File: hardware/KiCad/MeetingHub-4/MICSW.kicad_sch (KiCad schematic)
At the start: 13 parts, among them K1 Select NB1, K2 Select NB2, K3 Select NB3, K4 Select NB4, SW1 MUTE, SW2 Select NB1, SW3 Select NB2, SW4 Select NB3, SW5 Select NB4

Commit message: jlcpcb production  W2026080810364558  PCB/PCBA
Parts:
- SW1, SW2, SW3, SW4, SW5: footprint Connector_JST:JST_XH_B2B-XH-A_1x02_P2.50mm_Vertical -> MeetingHub-4:SW_SHOUHAN_TS665ZJ
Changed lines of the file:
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@@
       (effects (font (size 1.27 1.27)))
     )
-    (property "Footprint" "Connector_JST:JST_XH_B2B-XH-A_1x02_P2.50mm_Vertical" (at 95.25 39.37 0)
+    (property "Footprint" "MeetingHub-4:SW_SHOUHAN_TS665ZJ" (at 95.25 39.37 0)
       (effects (font (size 1.27 1.27)) hide)
     )
@@
       (effects (font (size 1.27 1.27)))
     )
-    (property "Footprint" "Connector_JST:JST_XH_B2B-XH-A_1x02_P2.50mm_Vertical" (at 59.69 30.48 0)
+    (property "Footprint" "MeetingHub-4:SW_SHOUHAN_TS665ZJ" (at 59.69 30.48 0)
       (effects (font (size 1.27 1.27)) hide)
     )
@@
       (effects (font (size 1.27 1.27)))
     )
-    (property "Footprint" "Connector_JST:JST_XH_B2B-XH-A_1x02_P2.50mm_Vertical" (at 95.25 80.01 0)
+    (property "Footprint" "MeetingHub-4:SW_SHOUHAN_TS665ZJ" (at 95.25 80.01 0)
       (effects (font (size 1.27 1.27)) hide)
     )
@@
       (effects (font (size 1.27 1.27)))
     )
-    (property "Footprint" "Connector_JST:JST_XH_B2B-XH-A_1x02_P2.50mm_Vertical" (at 95.25 160.02 0)
+    (property "Footprint" "MeetingHub-4:SW_SHOUHAN_TS665ZJ" (at 95.25 160.02 0)
       (effects (font (size 1.27 1.27)) hide)
     )
@@
       (effects (font (size 1.27 1.27)))
     )
-    (property "Footprint" "Connector_JST:JST_XH_B2B-XH-A_1x02_P2.50mm_Vertical" (at 95.25 119.38 0)
-      (effects (font (size 1.27 1.27)) hide)
-    )
+    (property "Footprint" "MeetingHub-4:SW_SHOUHAN_TS665ZJ" (at 95.25 119.38 0)
+      (effects (font (size 1.27 1.27)) hide)
+    )

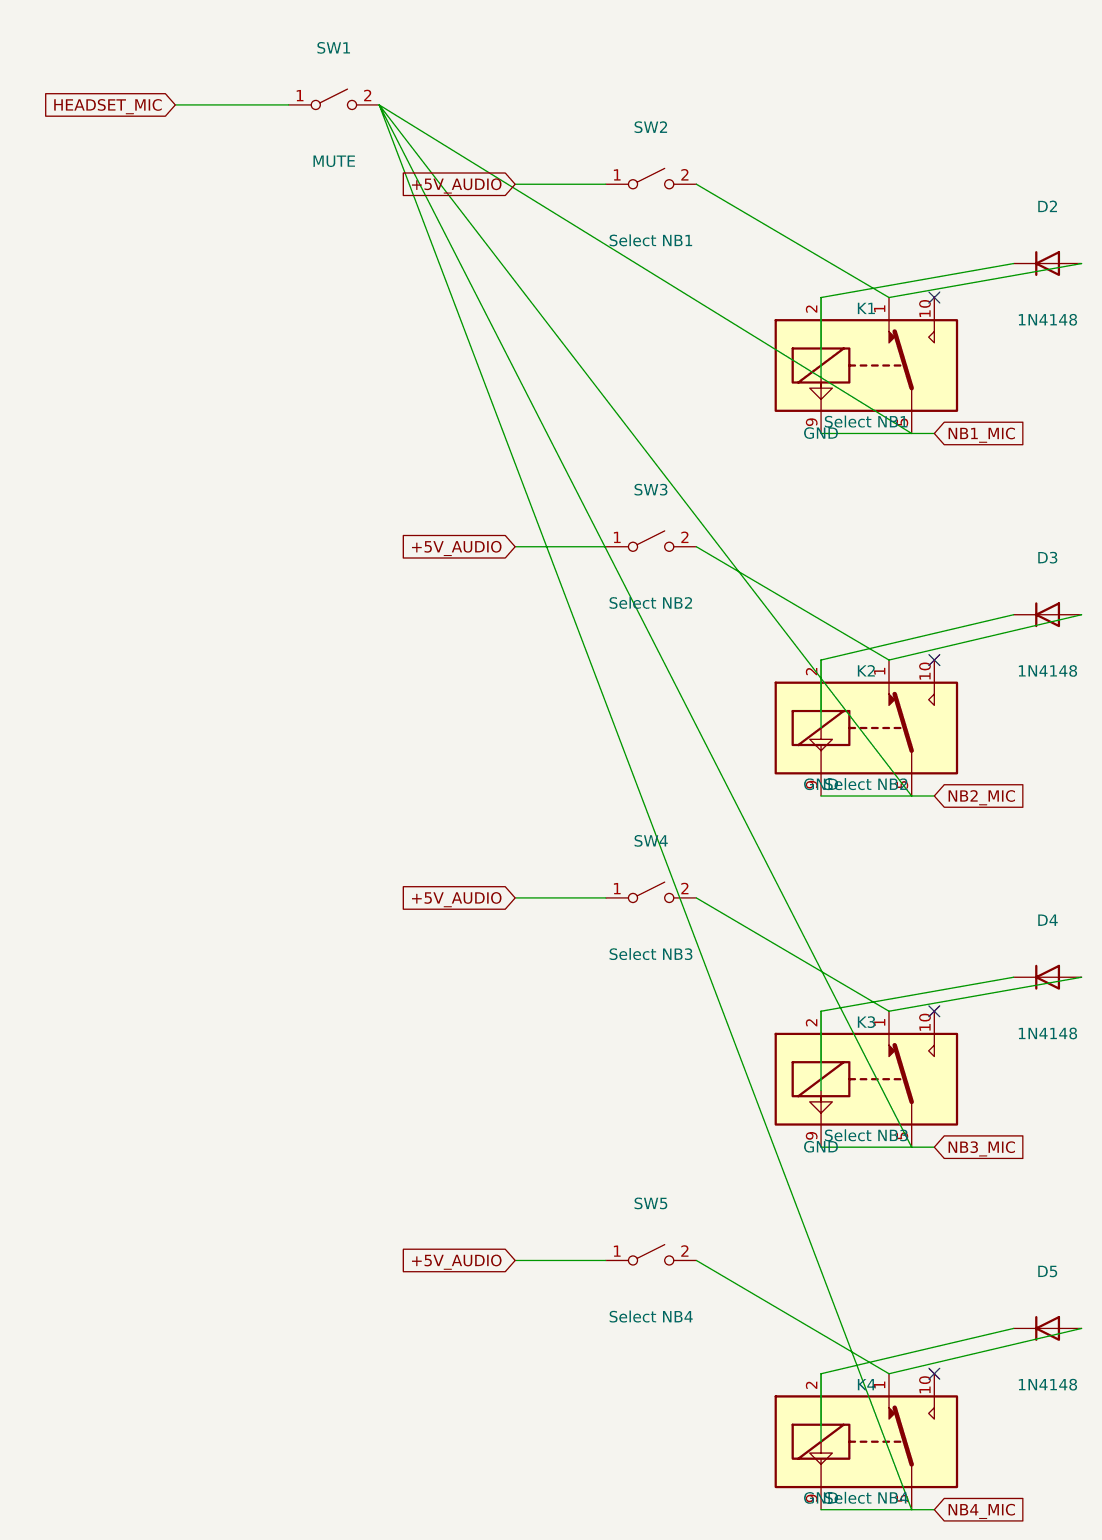
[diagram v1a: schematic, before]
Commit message: Rascunho projeto após fabricação com prblemas
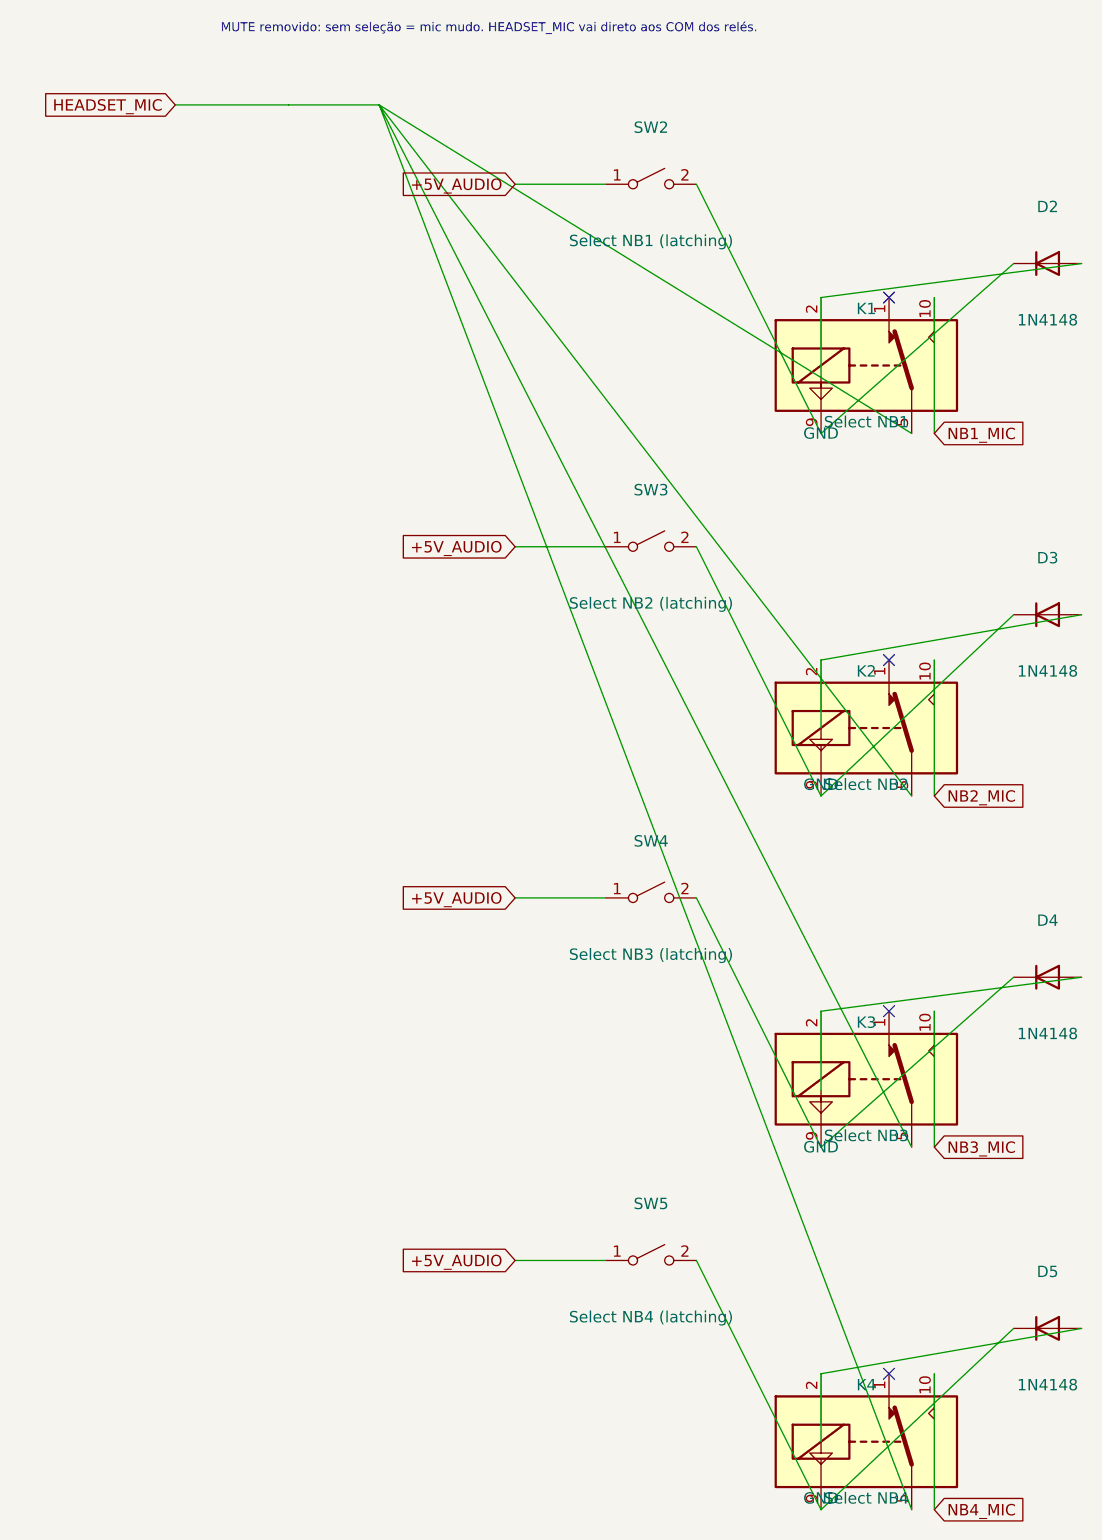
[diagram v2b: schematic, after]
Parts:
- removed SW1: MUTE, MeetingHub-4:SW_SHOUHAN_TS665ZJ, symbol Switch:SW_SPST
- SW2: value Select NB1 -> Select NB1 (latching); footprint MeetingHub-4:SW_SHOUHAN_TS665ZJ -> MeetingHub-4:SW_PushLock_PS-22F03
- SW3: value Select NB2 -> Select NB2 (latching); footprint MeetingHub-4:SW_SHOUHAN_TS665ZJ -> MeetingHub-4:SW_PushLock_PS-22F03
- SW4: value Select NB3 -> Select NB3 (latching); footprint MeetingHub-4:SW_SHOUHAN_TS665ZJ -> MeetingHub-4:SW_PushLock_PS-22F03
- SW5: value Select NB4 -> Select NB4 (latching); footprint MeetingHub-4:SW_SHOUHAN_TS665ZJ -> MeetingHub-4:SW_PushLock_PS-22F03
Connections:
- net GND: now also D2.2 (A), D3.2 (A), D4.2 (A), D5.2 (A); no longer D2.1 (K), D3.1 (K), D4.1 (K), D5.1 (K)
- net HEADSET_MIC: now also K1.5, K1.6, K2.5, K2.6, K3.5, K3.6, K4.5, K4.6
- net NB1_MIC: now also K1.10; no longer K1.9
- net NB2_MIC: now also K2.10; no longer K2.9
- net NB3_MIC: now also K3.10; no longer K3.9
- net NB4_MIC: now also K4.10; no longer K4.9
- new net: D2.1 (K), K1.9, SW2.2 (B)
- new net: D3.1 (K), K2.9, SW3.2 (B)
- new net: D4.1 (K), K3.9, SW4.2 (B)
- new net: D5.1 (K), K4.9, SW5.2 (B)
- now unconnected: K1.1, K2.1, K3.1, K4.1
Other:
- note added: "MUTE removido: sem seleção = mic mudo. HEADSET_MIC vai direto aos COM dos relés."
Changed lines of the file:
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@@
 (kicad_sch (version 20230121) (generator eeschema)
   (paper "A4")
-  (wire (pts (xy 100.33 160.02) (xy 121.92 172.72))
-    (stroke (width 0) (type default))
-  )
-  (no_connect (at 127 52.07))
-  (no_connect (at 127 92.71))
-  (no_connect (at 127 132.08))
-  (no_connect (at 127 172.72))
-  (wire (pts (xy 114.3 107.95) (xy 127 107.95))
-    (stroke (width 0) (type default))
-  )
-  (wire (pts (xy 114.3 187.96) (xy 127 187.96))
-    (stroke (width 0) (type default))
-  )
-  (wire (pts (xy 135.89 87.63) (xy 114.3 92.71))
-    (stroke (width 0) (type default))
-  )
-  (wire (pts (xy 143.51 128.27) (xy 121.92 132.08))
+  (wire (pts (xy 100.33 160.02) (xy 114.3 187.96))
+    (stroke (width 0) (type default))
+  )
+  (no_connect (at 121.92 52.07))
+  (no_connect (at 121.92 92.71))
+  (no_connect (at 121.92 132.08))
+  (no_connect (at 121.92 172.72))
+  (wire (pts (xy 127 92.71) (xy 127 107.95))
+    (stroke (width 0) (type default))
+  )
+  (wire (pts (xy 127 172.72) (xy 127 187.96))
+    (stroke (width 0) (type default))
+  )
+  (wire (pts (xy 135.89 87.63) (xy 114.3 107.95))
+    (stroke (width 0) (type default))
+  )
+  (wire (pts (xy 143.51 128.27) (xy 114.3 132.08))
     (stroke (width 0) (type default))
   )
@@
     (stroke (width 0) (type default))
   )
-  (wire (pts (xy 100.33 39.37) (xy 121.92 52.07))
+  (wire (pts (xy 100.33 39.37) (xy 114.3 67.31))
     (stroke (width 0) (type default))
   )
@@
     (stroke (width 0) (type default))
   )
+  (wire (pts (xy 54.61 30.48) (xy 64.77 30.48))
+    (stroke (width 0) (type default))
+  )
   (wire (pts (xy 114.3 132.08) (xy 114.3 140.97))
     (stroke (width 0) (type default))
@@
     (stroke (width 0) (type default))
   )
-  (wire (pts (xy 114.3 67.31) (xy 127 67.31))
-    (stroke (width 0) (type default))
-  )
-  (wire (pts (xy 114.3 147.32) (xy 127 147.32))
+  (wire (pts (xy 127 52.07) (xy 127 67.31))
+    (stroke (width 0) (type default))
+  )
+  (wire (pts (xy 127 132.08) (xy 127 147.32))
     (stroke (width 0) (type default))
   )
@@
     (stroke (width 0) (type default))
   )
-  (wire (pts (xy 135.89 48.26) (xy 114.3 52.07))
-    (stroke (width 0) (type default))
-  )
-  (wire (pts (xy 143.51 48.26) (xy 121.92 52.07))
-    (stroke (width 0) (type default))
-  )
-  (wire (pts (xy 135.89 128.27) (xy 114.3 132.08))
+  (wire (pts (xy 135.89 48.26) (xy 114.3 67.31))
+    (stroke (width 0) (type default))
+  )
+  (wire (pts (xy 143.51 48.26) (xy 114.3 52.07))
+    (stroke (width 0) (type default))
+  )
+  (wire (pts (xy 135.89 128.27) (xy 114.3 147.32))
     (stroke (width 0) (type default))
   )
@@
     (stroke (width 0) (type default))
   )
-  (wire (pts (xy 100.33 119.38) (xy 121.92 132.08))
-    (stroke (width 0) (type default))
-  )
-  (wire (pts (xy 135.89 167.64) (xy 114.3 172.72))
+  (wire (pts (xy 100.33 119.38) (xy 114.3 147.32))
+    (stroke (width 0) (type default))
+  )
+  (wire (pts (xy 135.89 167.64) (xy 114.3 187.96))
     (stroke (width 0) (type default))
   )
@@
     (stroke (width 0) (type default))
   )
-  (wire (pts (xy 143.51 167.64) (xy 121.92 172.72))
+  (wire (pts (xy 143.51 167.64) (xy 114.3 172.72))
     (stroke (width 0) (type default))
   )
@@
     (stroke (width 0) (type default))
   )
-  (wire (pts (xy 100.33 80.01) (xy 121.92 92.71))
-    (stroke (width 0) (type default))
-  )
-  (wire (pts (xy 143.51 87.63) (xy 121.92 92.71))
+  (wire (pts (xy 100.33 80.01) (xy 114.3 107.95))
+    (stroke (width 0) (type default))
+  )
+  (wire (pts (xy 143.51 87.63) (xy 114.3 92.71))
     (stroke (width 0) (type default))
   )
@@
       (effects (font (size 1.27 1.27)))
     )
-    (property "Value" "Select NB1" (at 95.25 45.72 0)
-      (effects (font (size 1.27 1.27)))
-    )
-    (property "Footprint" "MeetingHub-4:SW_SHOUHAN_TS665ZJ" (at 95.25 39.37 0)
+    (property "Value" "Select NB1 (latching)" (at 95.25 45.72 0)
+      (effects (font (size 1.27 1.27)))
+    )
+    (property "Footprint" "MeetingHub-4:SW_PushLock_PS-22F03" (at 95.25 39.37 0)
       (effects (font (size 1.27 1.27)) hide)
     )
@@
     )
   )
-  (symbol (lib_id "Switch:SW_SPST") (at 59.69 30.48 0) (unit 1)
-    (in_bom yes) (on_board yes) (dnp no)
-    (property "Reference" "SW1" (at 59.69 24.13 0)
-      (effects (font (size 1.27 1.27)))
-    )
-    (property "Value" "MUTE" (at 59.69 36.83 0)
-      (effects (font (size 1.27 1.27)))
-    )
-    (property "Footprint" "MeetingHub-4:SW_SHOUHAN_TS665ZJ" (at 59.69 30.48 0)
-      (effects (font (size 1.27 1.27)) hide)
-    )
-    (property "Datasheet" "" (at 59.69 30.48 0)
-      (effects (font (size 1.27 1.27)) hide)
-    )
-    (pin "1")
-    (pin "2")
-    (instances
-      (project "MeetingHub-4"
-        (path "/8b7deae6-c6d2-463d-9623-40608a842bd8/1a2b3c4d-0004-4a1a-8a1a-000000000004"
-          (reference "SW1") (unit 1)
-        )
-      )
-    )
+  (text "MUTE removido: sem seleção = mic mudo. HEADSET_MIC vai direto aos COM dos relés."
+    (at 47.0 22.0 0) (effects (font (size 1.0 1.0)) (justify left))
   )
   (symbol (lib_id "Device:D") (at 139.7 128.27 0) (unit 1)
@@
       (effects (font (size 1.27 1.27)))
     )
-    (property "Value" "Select NB2" (at 95.25 86.36 0)
-      (effects (font (size 1.27 1.27)))
-    )
-    (property "Footprint" "MeetingHub-4:SW_SHOUHAN_TS665ZJ" (at 95.25 80.01 0)
+    (property "Value" "Select NB2 (latching)" (at 95.25 86.36 0)
+      (effects (font (size 1.27 1.27)))
+    )
+    (property "Footprint" "MeetingHub-4:SW_PushLock_PS-22F03" (at 95.25 80.01 0)
       (effects (font (size 1.27 1.27)) hide)
     )
@@
       (effects (font (size 1.27 1.27)))
     )
-    (property "Value" "Select NB4" (at 95.25 166.37 0)
-      (effects (font (size 1.27 1.27)))
-    )
-    (property "Footprint" "MeetingHub-4:SW_SHOUHAN_TS665ZJ" (at 95.25 160.02 0)
+    (property "Value" "Select NB4 (latching)" (at 95.25 166.37 0)
+      (effects (font (size 1.27 1.27)))
+    )
+    (property "Footprint" "MeetingHub-4:SW_PushLock_PS-22F03" (at 95.25 160.02 0)
       (effects (font (size 1.27 1.27)) hide)
     )
@@
       (effects (font (size 1.27 1.27)))
     )
-    (property "Value" "Select NB3" (at 95.25 125.73 0)
-      (effects (font (size 1.27 1.27)))
-    )
-    (property "Footprint" "MeetingHub-4:SW_SHOUHAN_TS665ZJ" (at 95.25 119.38 0)
-      (effects (font (size 1.27 1.27)) hide)
-    )
+    (property "Value" "Select NB3 (latching)" (at 95.25 125.73 0)
+      (effects (font (size 1.27 1.27)))
+    )
+    (property "Footprint" "MeetingHub-4:SW_PushLock_PS-22F03" (at 95.25 119.38 0)
+      (effects (font (size 1.27 1.27)) hide)
+    )
